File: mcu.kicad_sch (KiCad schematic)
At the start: 1 part, among them U1 ESP32-S3-WROOM-1

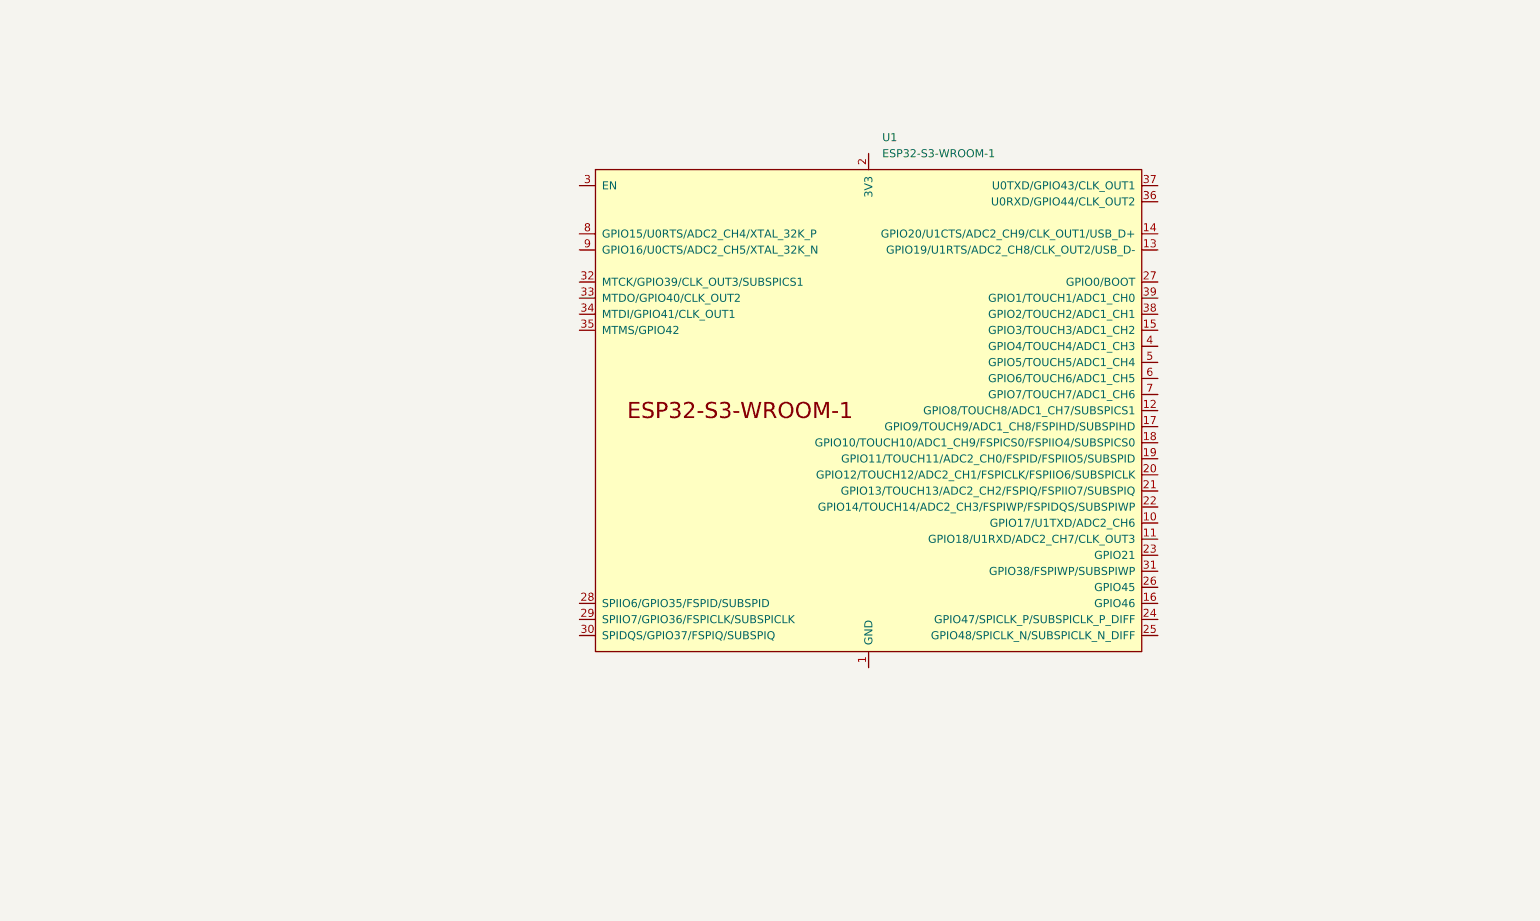
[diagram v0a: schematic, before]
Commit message: almost done
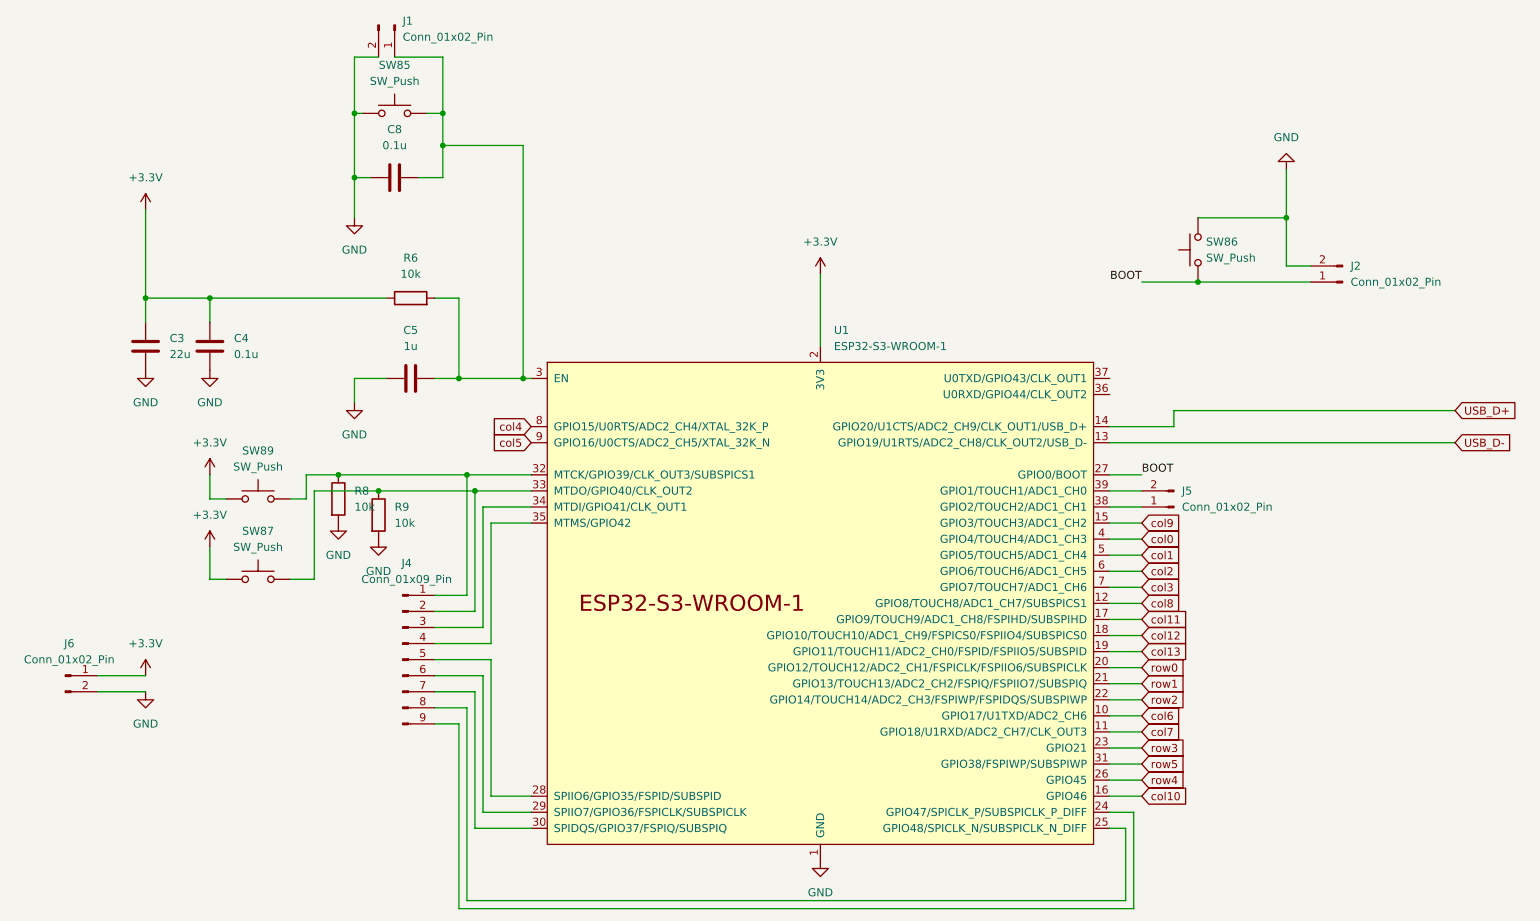
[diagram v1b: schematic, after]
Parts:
- added C3: 22u, Capacitor_SMD:C_0805_2012Metric_Pad1.18x1.45mm_HandSolder, symbol Device:C
- added C4, C8: 0.1u, Capacitor_SMD:C_0805_2012Metric_Pad1.18x1.45mm_HandSolder, symbol Device:C
- added C5: 1u, Capacitor_SMD:C_0805_2012Metric_Pad1.18x1.45mm_HandSolder, symbol Device:C
- added J1, J2, J5, J6: Conn_01x02_Pin, Connector_PinHeader_2.54mm:PinHeader_1x02_P2.54mm_Vertical, symbol Connector:Conn_01x02_Pin
- added J4: Conn_01x09_Pin, Connector_PinHeader_2.54mm:PinHeader_1x09_P2.54mm_Vertical, symbol Connector:Conn_01x09_Pin
- added R6, R8, R9: 10k, Resistor_SMD:R_0805_2012Metric_Pad1.20x1.40mm_HandSolder, symbol Device:R
- added SW85, SW86, SW87, SW89: SW_Push, Button_Switch_THT:SW_PUSH_6mm, symbol Switch:SW_Push
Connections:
- net GND: now reaches U1.1 (GND), U1.40 (GND), U1.41 (GND)
- net GND: now also C3.2, C4.2, C5.1, C8.1, J1.2 (Pin_2), J2.2 (Pin_2), J6.2 (Pin_2), R8.2, R9.2, SW85.1, SW86.2
- net col6: now reaches U1.10 (GPIO17/U1TXD/ADC2_CH6)
- net col7: now reaches U1.11 (GPIO18/U1RXD/ADC2_CH7/CLK_OUT3)
- net col8: now reaches U1.12 (GPIO8/TOUCH8/ADC1_CH7/SUBSPICS1)
- net USB_D-: now reaches U1.13 (GPIO19/U1RTS/ADC2_CH8/CLK_OUT2/USB_D-)
- net USB_D+: now reaches U1.14 (GPIO20/U1CTS/ADC2_CH9/CLK_OUT1/USB_D+)
- net col9: now reaches U1.15 (GPIO3/TOUCH3/ADC1_CH2)
- net col10: now reaches U1.16 (GPIO46)
- net col11: now reaches U1.17 (GPIO9/TOUCH9/ADC1_CH8/FSPIHD/SUBSPIHD)
- net col12: now reaches U1.18 (GPIO10/TOUCH10/ADC1_CH9/FSPICS0/FSPIIO4/SUBSPICS0)
- net col13: now reaches U1.19 (GPIO11/TOUCH11/ADC2_CH0/FSPID/FSPIIO5/SUBSPID)
- net +3.3V: now reaches U1.2 (3V3)
- net +3.3V: now also C3.1, C4.1, J6.1 (Pin_1), R6.1, SW87.1, SW89.1
- net row0: now reaches U1.20 (GPIO12/TOUCH12/ADC2_CH1/FSPICLK/FSPIIO6/SUBSPICLK)
- net row1: now reaches U1.21 (GPIO13/TOUCH13/ADC2_CH2/FSPIQ/FSPIIO7/SUBSPIQ)
- net row2: now reaches U1.22 (GPIO14/TOUCH14/ADC2_CH3/FSPIWP/FSPIDQS/SUBSPIWP)
- net row3: now reaches U1.23 (GPIO21)
- net at U1.24 (GPIO47/SPICLK_P/SUBSPICLK_P_DIFF): now also J4.9 (Pin_9)
- net at U1.25 (GPIO48/SPICLK_N/SUBSPICLK_N_DIFF): now also J4.8 (Pin_8)
- net row4: now reaches U1.26 (GPIO45)
- net BOOT: now reaches U1.27 (GPIO0/BOOT)
- net BOOT: now also J2.1 (Pin_1), SW86.1
- net at U1.28 (SPIIO6/GPIO35/FSPID/SUBSPID): now also J4.5 (Pin_5)
- net at U1.29 (SPIIO7/GPIO36/FSPICLK/SUBSPICLK): now also J4.6 (Pin_6)
- net at U1.3 (EN): now also C5.2, C8.2, J1.1 (Pin_1), R6.2, SW85.2
- net at U1.30 (SPIDQS/GPIO37/FSPIQ/SUBSPIQ): now also J4.7 (Pin_7)
- net row5: now reaches U1.31 (GPIO38/FSPIWP/SUBSPIWP)
- net at U1.32 (MTCK/GPIO39/CLK_OUT3/SUBSPICS1): now also J4.1 (Pin_1), R8.1, SW89.2
- net at U1.33 (MTDO/GPIO40/CLK_OUT2): now also J4.2 (Pin_2), R9.1, SW87.2
- net at U1.34 (MTDI/GPIO41/CLK_OUT1): now also J4.3 (Pin_3)
- net at U1.35 (MTMS/GPIO42): now also J4.4 (Pin_4)
- net at U1.38 (GPIO2/TOUCH2/ADC1_CH1): now also J5.1 (Pin_1)
- net at U1.39 (GPIO1/TOUCH1/ADC1_CH0): now also J5.2 (Pin_2)
- net col0: now reaches U1.4 (GPIO4/TOUCH4/ADC1_CH3)
- net col1: now reaches U1.5 (GPIO5/TOUCH5/ADC1_CH4)
- net col2: now reaches U1.6 (GPIO6/TOUCH6/ADC1_CH5)
- net col3: now reaches U1.7 (GPIO7/TOUCH7/ADC1_CH6)
- net col4: now reaches U1.8 (GPIO15/U0RTS/ADC2_CH4/XTAL_32K_P)
- net col5: now reaches U1.9 (GPIO16/U0CTS/ADC2_CH5/XTAL_32K_N)
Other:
- moved on the sheet: U1
